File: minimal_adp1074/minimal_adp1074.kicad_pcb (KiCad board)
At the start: 4 copper layers, 43.2 x 30.5 mm, 5 parts, among them T1 PL160X9-102L-BLD, U1 ADP1074ACCZ-R7

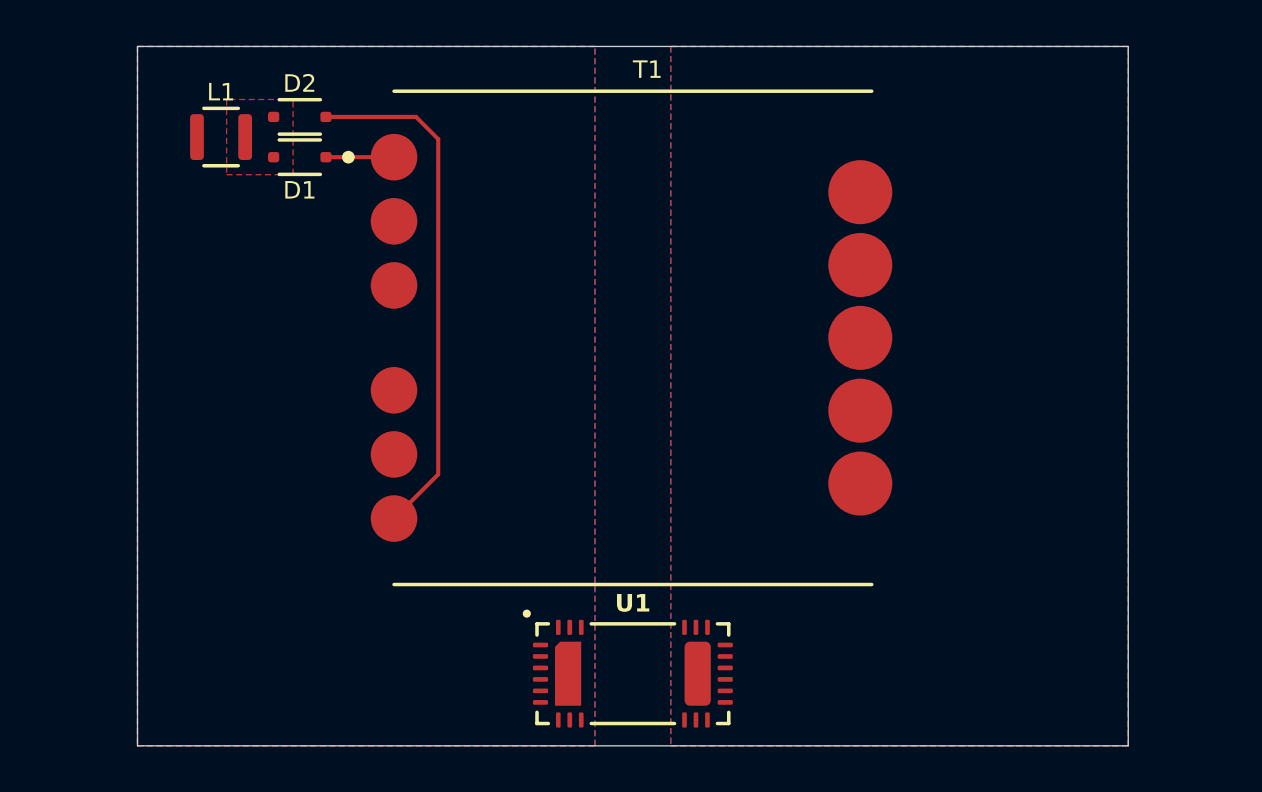
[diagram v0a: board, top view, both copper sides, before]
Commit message: backup
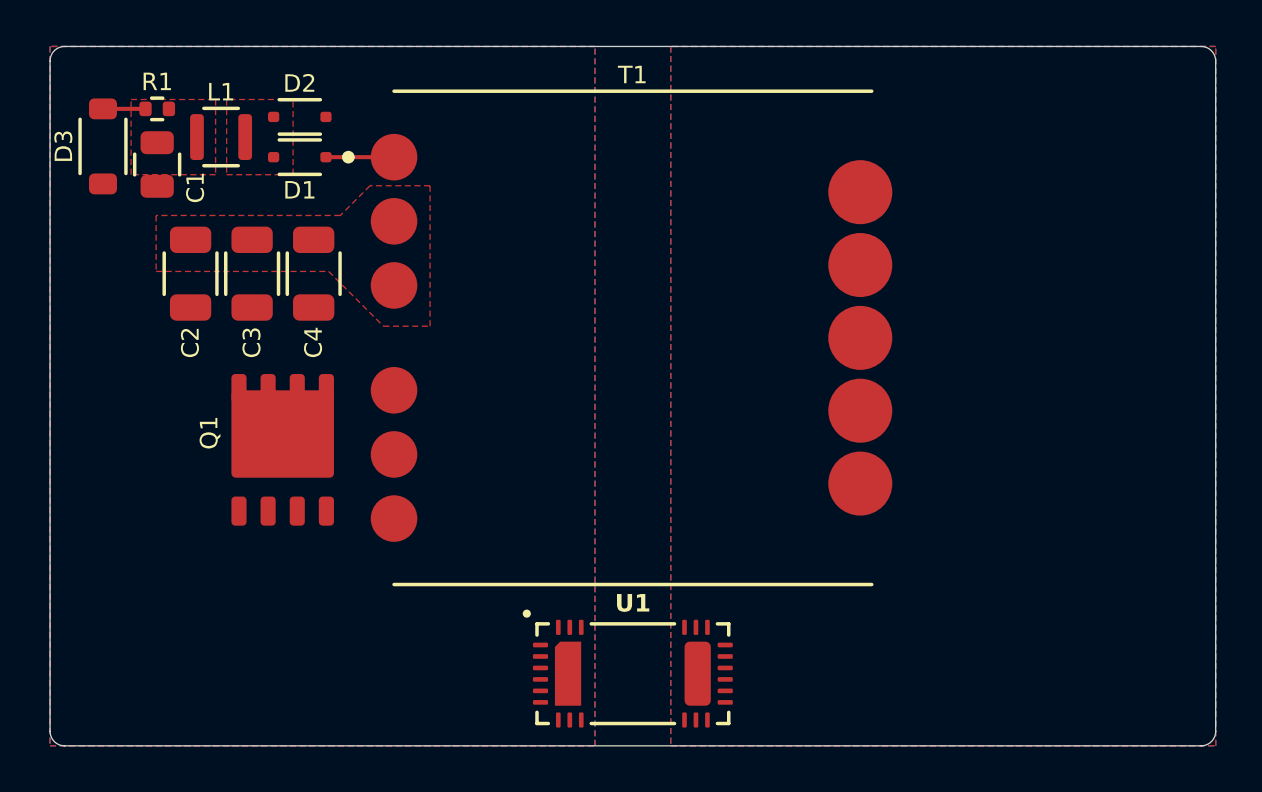
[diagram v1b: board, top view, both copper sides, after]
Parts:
- added C1: 2.2 µF, capacitor_footprints:C_0805_2012Metric, F.Cu at (131.7, 81.3)
- added C2: 2.2 µF, capacitor_footprints:C_1206_3216Metric, F.Cu at (133.1, 86.1)
- added C3: 2.2 µF, capacitor_footprints:C_1206_3216Metric, F.Cu at (135.8, 86.1)
- added C4: 2.2 µF, capacitor_footprints:C_1206_3216Metric, F.Cu at (138.5, 86.1)
- added D3: 11.0 V, diode_footprints:SOD_123, F.Cu at (129.3, 80.6)
- added Q1: 80 V, transistor_footprints:PowerPAK SO-8 Single, F.Cu at (137.1, 93.8)
- added R1: 100 Ω, resistor_footprints:R_0402_1005Metric, F.Cu at (131.7, 78.9)
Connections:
- D2 pad 2: Net-(D2-Pad2) -> GND
- L1 pad 2: unconnected-(L1-Pad2) -> /V_AUX
- T1 pad 6: Net-(D2-Pad2) -> GND
- U1 pad 1: unconnected-(U1-NGATE-Pad1) -> /N_GATE
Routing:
- net Net-(D2-Pad2): track 22.6 -> 0.00 mm
- net Net-(D3-Pad1): track 0.00 -> 1.85 mm
- added copper zone on F.Cu, net /VIN
- added copper zone on F.Cu, net /V_AUX
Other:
- board size 43.2 x 30.5 mm -> 50.8 x 30.5 mm
